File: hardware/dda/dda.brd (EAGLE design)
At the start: 160 x 100 mm, 63 parts, among them IC1 74LS132D, K1 CP1-12V, T1 BC847, T2 BC847, T3 BC847, T4 BC847, T5 BC847, T6 BC847, T7 BC847, T8 BC847, T9 BC847

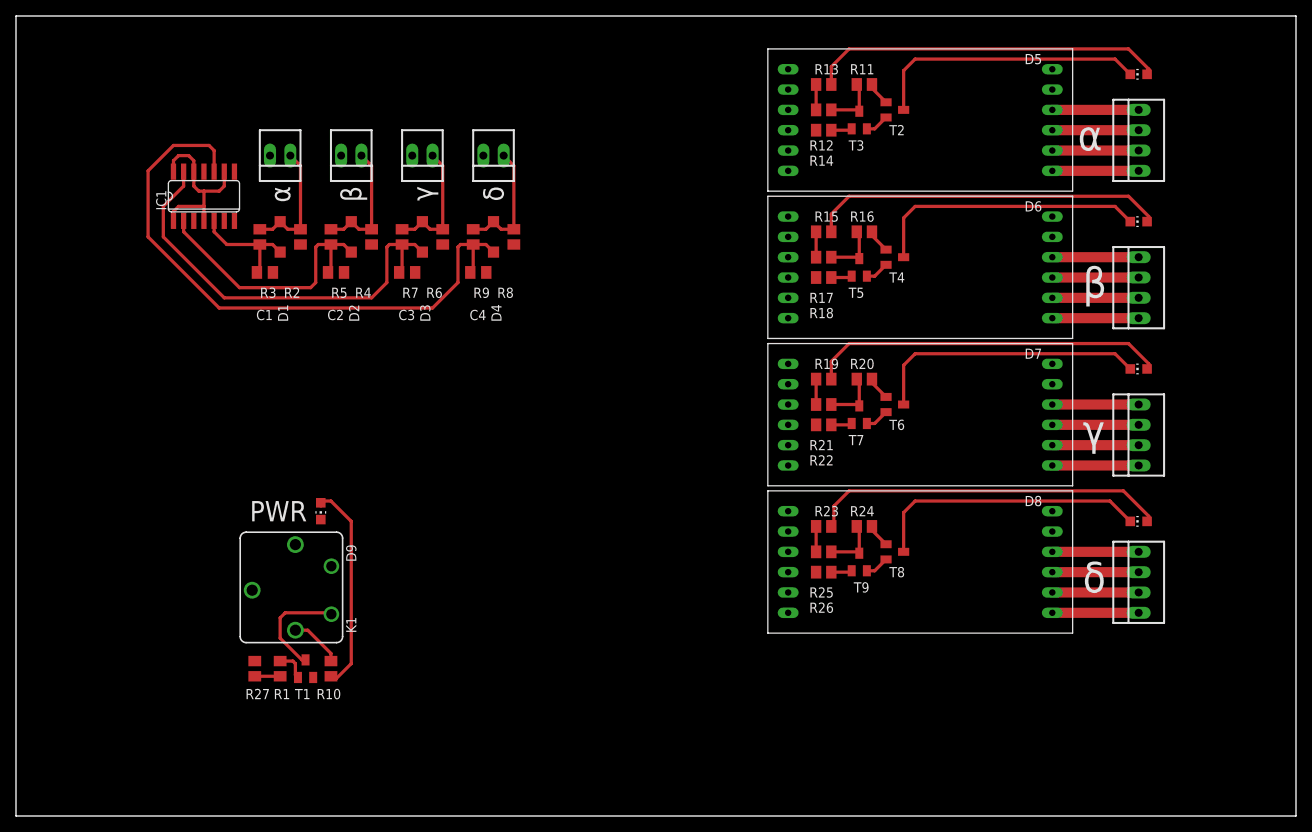
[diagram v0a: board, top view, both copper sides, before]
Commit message: DDA board routed v1.0b
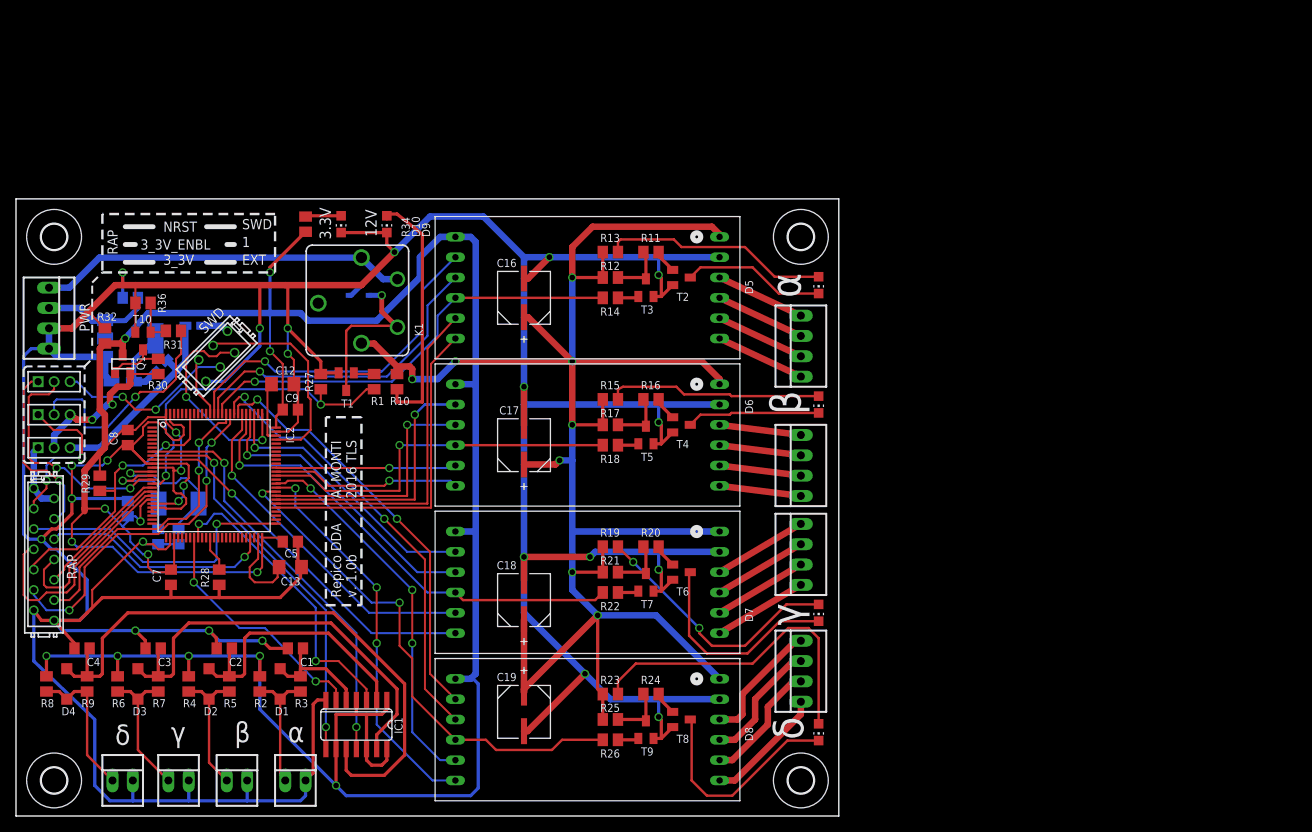
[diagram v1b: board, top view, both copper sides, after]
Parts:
- removed A_MOTOR, B_MOTOR, D_MOTOR, G_MOTOR: 22-23-2041, con-molex:22-23-2041
- removed D, G: STEPPER, stepper_module:STEPPER
- removed ENDSTOP_A, ENDSTOP_B, ENDSTOP_D, ENDSTOP_G: (no value), con-molex:22-23-2021
- added C10, C11: 18p, rcl:C0805
- added C12, C13: 2.2u, rcl:C1206
- added C14, C5, C6, C7, C8, C9: 100n, rcl:C0805
- added C15: 10u, rcl:CT3216
- added C16, C17, C18, C19: 220u, Panasonic-EEEFT_EEEH:CAPAE660X800N
- added D10: RED, led:CHIP-LED0805
- added D11: BAT60JFILM, diode:SOD323_ST
- added H1, H2, H3, H4: (no value), holes:3,2
- added IC2: STM32F407VGT, micro-stm_v2:LQFP100
- added IC3: LD1117, v-reg:SOT223
- added JP1, JP2, JP3: (no value), pinhead-2:1X03M
- added MOTOR_A, MOTOR_B, MOTOR_D, MOTOR_G, PWR: (no value), con-molex:22-23-2041
- added Q1: FDN304P, transistor-power:SUPER-SOT3
- added R28, R29, R30: 10K, rcl:M0805
- added R31: 4K7, rcl:M0805
- added R32, R36: 20K, rcl:M0805
- added R33, R35: 0R, rcl:R0805W
- added R34: 100R, rcl:M0805
- added RAP: (no value), con-amp-micromatch:MICROMATCH-14
- added STEPPER_D, STEPPER_G: REPICO_STEPPER, stepper_module:REPICO_STEPPER
- added SWD: (no value), con-amp-micromatch:MICROMATCH-6
- added T10: BC847, transistor:SOT23
- added X1, X2, X3, X4: 22-23-2021, con-molex:22-23-2021
- added Y1: 8MHz, Simplex-FreqCtrl:CRYSTAL-SMD-5X3.2
- C1, C4: value 10u -> 100n; device rcl:C0805K -> rcl:C0805
- C2, C3: device rcl:C0805K -> rcl:C0805
- D5, D6, D7, D8: value (none) -> YELLOW
- D9: value (none) -> RED
- IC1: value 74LS132D -> CD74HC32M
- R1: value 3K3 -> 4K7
- R10: value 330 -> 560R
- R11, R13, R15, R16, R19, R20, R23, R24: value 470 -> 560R
- R12, R17, R21, R25: value 12K -> 10K
- R27: value 3K3 -> 20K
- STEPPER_A, STEPPER_B: value STEPPER -> REPICO_STEPPER; device stepper_module:STEPPER -> stepper_module:REPICO_STEPPER
- moved R8 80.8 mm to (3.81, 16.5), turned to 90 degrees
- moved D4 77.3 mm to (6.35, 16.5), turned to 270 degrees
- moved R9 73.8 mm to (8.89, 16.5), turned to 90 degrees
- moved R6 69.1 mm to (12.7, 16.5), turned to 90 degrees
- moved IC1 68.7 mm to (42.5, 11.4), turned to 180 degrees
- moved C4 68.3 mm to (8.26, 21.0), turned to 180 degrees
- moved D3 66.2 mm to (15.2, 16.5), turned to 270 degrees
- moved R7 63.7 mm to (17.8, 16.5), turned to 90 degrees
- moved R4 60.4 mm to (21.6, 16.5), turned to 90 degrees
- moved D2 58.6 mm to (24.1, 16.5), turned to 270 degrees
- moved R5 57.3 mm to (26.7, 16.5), turned to 90 degrees
- moved C3 56.7 mm to (17.1, 21.0), turned to 180 degrees
- moved R2 56.1 mm to (30.5, 16.5), turned to 90 degrees
- moved R3 56.1 mm to (35.6, 16.5), turned to 90 degrees
- moved D1 55.9 mm to (33.0, 16.5), turned to 270 degrees
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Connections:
- removed net 12V_ENABLE: R1.1, R27.2
- removed net ENDSTOP_A: IC1.6
- removed net ENDSTOP_B: IC1.3
- removed net ENDSTOP_D: IC1.8
- removed net ENDSTOP_G: IC1.11
- removed net N$10: G.OUT1A, G_MOTOR.2
- removed net N$11: G.OUT2A, G_MOTOR.3
- removed net N$12: G.OUT2B, G_MOTOR.4
- removed net N$13: D.OUT1B, D_MOTOR.1
- removed net N$14: D.OUT1A, D_MOTOR.2
- removed net N$15: D.OUT2A, D_MOTOR.3
- removed net N$16: D.OUT2B, D_MOTOR.4
- removed net N$19: D1.A, ENDSTOP_A.1, R2.1, R3.1
- removed net N$21: D2.A, ENDSTOP_B.1, R4.1, R5.1
- removed net N$23: D3.A, ENDSTOP_G.1, R6.1, R7.1
- removed net N$25: D4.A, ENDSTOP_D.1, R8.1, R9.1
- removed net N$4: A_MOTOR.4, STEPPER_A.OUT2B
- removed net N$6: B_MOTOR.2, STEPPER_B.OUT1A
- removed net N$7: B_MOTOR.3, STEPPER_B.OUT2A
- removed net N$8: B_MOTOR.4, STEPPER_B.OUT2B
- new net 12V_ENBL: IC2.15, R1.1, R27.2
- new net 3_3V_ENBL: JP2.2, R31.2
- new net A_ENDST: IC1.6, IC2.33
- new net A_ENDSW: D1.A, R2.1, R3.1, X1.1
- new net A_OUT1A: MOTOR_A.2, STEPPER_A.OUT1A
- new net A_OUT1B: MOTOR_A.1, STEPPER_A.OUT1B
- new net A_OUT2A: MOTOR_A.3, STEPPER_A.OUT2A
- new net A_OUT2B: MOTOR_A.4, STEPPER_A.OUT2B
- new net BOOT1: IC2.37, R28.2
- new net B_ENDST: IC1.3, IC2.34
- new net B_ENDSW: D2.A, R4.1, R5.1, X2.1
- new net B_OUT1A: MOTOR_B.2, STEPPER_B.OUT1A
- new net B_OUT1B: MOTOR_B.1, STEPPER_B.OUT1B
- new net B_OUT2A: MOTOR_B.3, STEPPER_B.OUT2A
- new net B_OUT2B: MOTOR_B.4, STEPPER_B.OUT2B
- new net D_ENDST: IC1.8, IC2.8
- new net D_ENDSW: D4.A, R8.1, R9.1, X4.1
- new net D_OUT1A: MOTOR_D.2, STEPPER_D.OUT1A
- new net D_OUT1B: MOTOR_D.1, STEPPER_D.OUT1B
- new net D_OUT2A: MOTOR_D.3, STEPPER_D.OUT2A
- new net D_OUT2B: MOTOR_D.4, STEPPER_D.OUT2B
- new net EXT_3_3V: JP3.3, R33.2, R35.2
- new net G_ENDST: IC1.11, IC2.7
- new net G_ENDSW: D3.A, R6.1, R7.1, X3.1
- new net G_OUT1A: MOTOR_G.2, STEPPER_G.OUT1A
- new net G_OUT1B: MOTOR_G.1, STEPPER_G.OUT1B
- new net G_OUT2A: MOTOR_G.3, STEPPER_G.OUT2A
- new net G_OUT2B: MOTOR_G.4, STEPPER_G.OUT2B
- new net NRST: IC2.14, JP1.2
- new net OSC_IN: C10.2, IC2.12, Y1.P$2
- new net OSC_OUT: C11.2, IC2.13, Y1.P$1
- new net RAP_3_3V: JP3.1, RAP.1, RAP.2
- new net RAP_BOOTSEL: IC2.94, R29.1, RAP.9
- new net RAP_ENBL: JP2.1, RAP.3
- new net RAP_INT0: IC2.16, RAP.10
- new net RAP_INT1: IC2.84, RAP.11
- new net RAP_INT2: IC2.85, RAP.12
- new net RAP_NRST: JP1.1, RAP.4
- new net SPI_MISO: IC2.17, RAP.8
- new net SPI_MOSI: IC2.18, RAP.7
- new net SPI_NSS: IC2.51, RAP.5
- new net SPI_SCK: IC2.47, RAP.6
- new net SUPPLY_3_3V: JP2.3, JP3.2, Q1.2, R30.2
- new net SUPPLY_5V: C14.1, IC3.3, PWR.2
- new net SWCLK: IC2.76, SWD.2
- new net SWDIO: IC2.72, SWD.3
- new net SWD_NRST: JP1.3, SWD.4
- new net SWO: IC2.89, SWD.5
- new net VBAT: IC2.6
- new net VCAP_1: C12.1, IC2.73
- new net VCAP_2: C13.1, IC2.49
- net 12V: now also C16.1, C17.1, C18.1, C19.1, STEPPER_D.VCC, STEPPER_G.VCC; no longer D.VCC, G.VCC
- net 3_3V: now also C5.1, C6.1, C7.1, C8.1, C9.1, IC2.100, IC2.11, IC2.19, IC2.21, IC2.22, IC2.28, IC2.50, IC2.75, Q1.3, R29.2, R32.2, R34.2, STEPPER_D.VDD, STEPPER_G.VDD; no longer D.VDD, G.VDD
- net A_DIR: now also IC2.55
- net A_DIS: now also IC2.86
- net A_MS1: now also IC2.88
- net A_MS2: now also IC2.87
- net A_STEP: now also IC2.56
- net B_DIR: now also IC2.64
- net B_DIS: now also IC2.63
- net B_MS1: now also IC2.57
- net B_MS2: now also IC2.58
- net B_STEP: now also IC2.65
- net D_DIR: now also IC2.60, STEPPER_D.DIR; no longer D.DIR
- net D_DIS: now also IC2.59, STEPPER_D.DIS; no longer D.DIS
- net D_MS1: now also IC2.82, STEPPER_D.MS1; no longer D.MS1
- net D_MS2: now also IC2.83, STEPPER_D.MS2; no longer D.MS2
- net D_STEP: now also IC2.61, STEPPER_D.STEP; no longer D.STEP
- net GND: now also C10.1, C11.1, C12.2, C13.2, C14.2, C15.-, C16.2, C17.2, C18.2, C19.2, C5.2, C6.2, C7.2, C8.2, C9.2, D10.C, IC2.10, IC2.20, IC2.27, IC2.74, IC2.99, IC3.1, PWR.3, PWR.4, R28.1, R32.1, R36.1, RAP.13, RAP.14, STEPPER_D.GND, STEPPER_G.GND, SWD.6, T10.2, X1.2, X2.2, X3.2, X4.2; no longer D.GND, ENDSTOP_A.2, ENDSTOP_B.2, ENDSTOP_D.2, ENDSTOP_G.2, G.GND
- net G_DIR: now also IC2.9, STEPPER_G.DIR; no longer G.DIR
- net G_DIS: now also IC2.80, STEPPER_G.DIS; no longer G.DIS
- net G_MS1: now also IC2.78, STEPPER_G.MS1; no longer G.MS1
- net G_MS2: now also IC2.79, STEPPER_G.MS2; no longer G.MS2
- net G_STEP: now also IC2.81, STEPPER_G.STEP; no longer G.STEP
- net N$1: now also Q1.1, R30.1, T10.3; no longer A_MOTOR.1, STEPPER_A.OUT1B
- net N$17: now also D11.A
- net N$2: now also R35.1, SWD.1; no longer A_MOTOR.2, STEPPER_A.OUT1A
- net N$3: now also R31.1, R36.2, T10.1; no longer A_MOTOR.3, STEPPER_A.OUT2A
- net N$5: now also D10.A, R34.1; no longer B_MOTOR.1, STEPPER_B.OUT1B
- net N$9: now also C15.+, IC3.4, R33.1; no longer G.OUT1B, G_MOTOR.1
- net SUPPLY_12V: now also D11.C, PWR.1
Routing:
- net GND: track 11.9 -> 640.0 mm, vias 0 -> 24
- net 3_3V: track 22.7 -> 387.7 mm, vias 0 -> 15
- net 12V: track 19.3 -> 228.3 mm, vias 0 -> 8
- net D_DIS: track 0.00 -> 64.1 mm, vias 0 -> 2
- net G_DIS: track 0.00 -> 59.6 mm, vias 0 -> 1
- net D_MS2: track 0.00 -> 56.0 mm, vias 0 -> 2
- net A_DIS: track 0.00 -> 55.8 mm, vias 0 -> 1
- net D_MS1: track 0.00 -> 52.9 mm, vias 0 -> 2
- net G_ENDST: track 0.00 -> 52.2 mm, vias 0 -> 2
- net SUPPLY_12V: track 0.00 -> 50.8 mm
- net D_ENDST: track 0.00 -> 49.7 mm, vias 0 -> 2
- net D_DIR: track 0.00 -> 48.9 mm, vias 0 -> 3
- net D_STEP: track 0.00 -> 47.4 mm, vias 0 -> 3
- net B_DIS: track 0.00 -> 47.3 mm, vias 0 -> 1
- net G_DIR: track 0.00 -> 46.9 mm, vias 0 -> 1
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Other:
- board size 160 x 100 mm -> 102.8 x 77.1 mm
- board text added: "-"
- board text added: "1"
- board text added: "12V"
- board text added: "2016 TLS"
- board text added: "3.3V"
- board text added: "3_3V"
- board text added: "3_3V_ENBL"
- board text added: "A. MONTI"
- board text added: "EXT"
- board text added: "Fit BAT60JFILM for supply protection"
- board text added: "NRST"
- board text added: "RAP"
- board text added: "Repico DDA"
- board text added: "SWD"
- board text added: "Y1"
- board text added: "v. 1.0b"
- board text removed: "PWR"
